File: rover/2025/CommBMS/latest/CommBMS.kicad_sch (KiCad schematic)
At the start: 22 parts

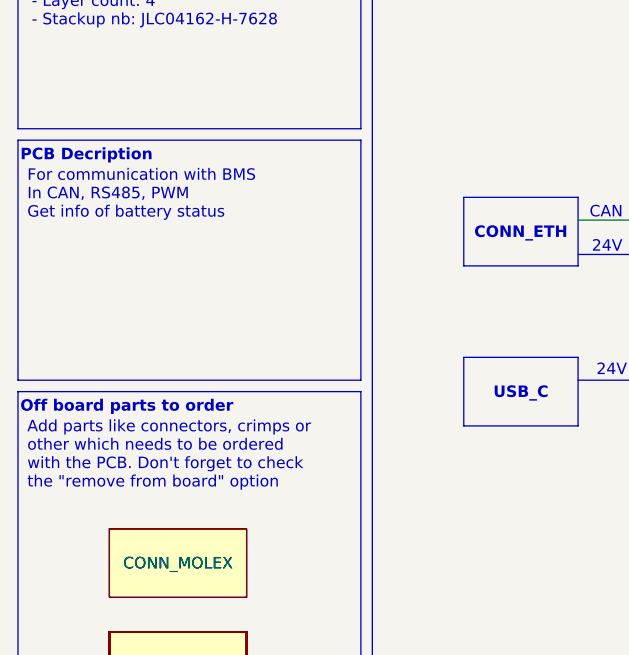
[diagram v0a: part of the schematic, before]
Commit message: BOM digikey
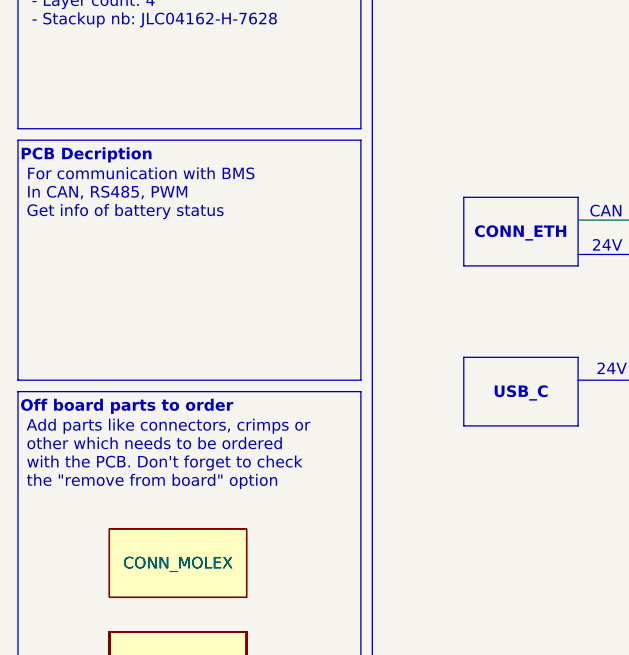
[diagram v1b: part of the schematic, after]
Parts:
- G1: Digikey TODO -> https://www.digikey.com/en/products/detail/molex/0039012080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
- G5: Digikey TODO -> https://www.digikey.com/en/products/detail/molex/0039000038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
